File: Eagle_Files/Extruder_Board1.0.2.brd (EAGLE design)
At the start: 39.6 x 46.5 mm, 22 parts, among them J1 10118192-0001LF, U1 CP2102N-A01-GQFN20

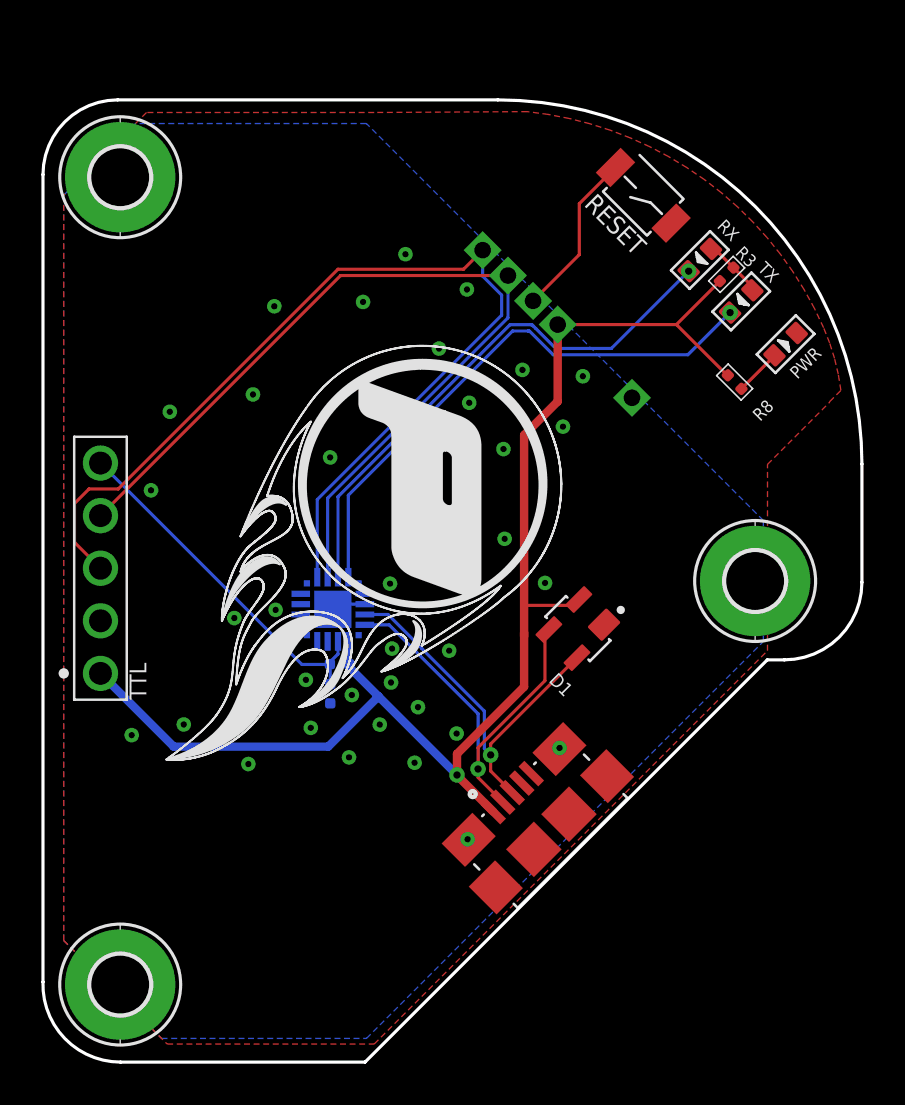
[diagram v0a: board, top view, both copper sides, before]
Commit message: pulled latest fixes from master
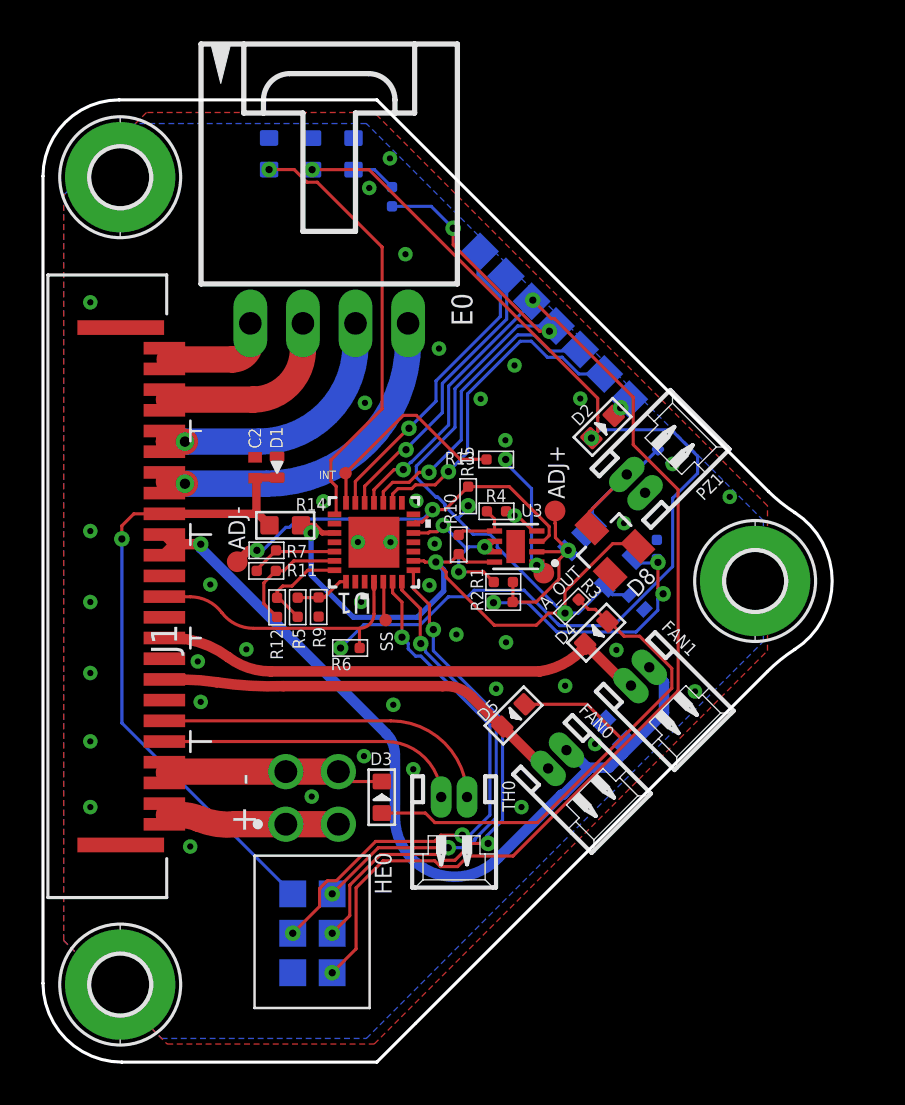
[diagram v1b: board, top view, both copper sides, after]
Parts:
- removed RESET: (no value), PiezoFFC:SEEED-SWITCH_SW2-2.6-3.0X2.5X1.2+0.4MM
- removed RX, TX: (no value), PiezoFFC:SEEED-LED_LED-0603
- removed TTL: JST-2.54MM_5P-2.54JST_2.54MM_5P_F, PiezoFFC:HDRVR5W64P254_1X5_1270X254X575B
- removed U$2: (no value), PiezoFFC:LOGO-PYR0BALL-SS-20MM
- added 5V, MISO, MOSI, RST, SCK: TPTP13SQ, PiezoFFC:TP13SQ
- added ADJ+, ADJ-, A_OUT: TPTP10R, PiezoFFC:TP10R
- added C1, C2: 0.1uF, PiezoFFC:CAPC1005X50
- added C3: 1uF, PiezoFFC:CAPC1609X80
- added D2, D3, D4, D5, ERR, TRG: (no value), PiezoFFC:SEEED-LED_LED-0603
- added D8: BAV199, PiezoFFC:SOT23
- added E0: C-GRID-04-70553, PiezoFFC:70553-04
- added FAN0, FAN1, PZ1, TH0: CON-MOLEX-2P-1.27MM048, PiezoFFC:53048-02
- added HE0: JST-2.54-2X2JST-DUPONT-2.54-2X2, PiezoFFC:HDRRAR4W64P254_2X2_556X736X556B
- added INT, SS: TPTP06R, testpad:TP06R
- added R10, R4: 10K, PiezoFFC:R0402
- added R11, R7: 220R, PiezoFFC:R0402
- added R12, R5: 330R, PiezoFFC:R0402
- added R13: 100R, PiezoFFC:R0402
- added R14: 0R, PiezoFFC:SEEED-RESISTOR_R0603
- added R15: 680R, PiezoFFC:R0402
- added R17: 3.3K, PiezoFFC:R0402
- added R19: 1M, PiezoFFC:R0402
- added R6: (no value), PiezoFFC:R0402
- added R9: 470R, PiezoFFC:R0402
- added SCL, SDA, ⏚: TPTP13SQ, testpad:TP13SQ
- added U2: MCP6001T-I/OTSOT-23-5_MC-L, PiezoFFC:SOT-23-5_MC-L
- added U3: LM358PWRDFN-8, PiezoFFC:SON50P200X200X60-9N
- +5V, GND, RST., RXD, TXD: value TP -> TPTP13SQ; device PiezoFFC:TP13SQ-HOLE -> testpad:TP13SQ
- D1: value SP0503BAHTG -> 1N4148DFN-1006-2; device PiezoFFC:SOT143 -> PiezoFFC:DIOC1006X70
- J1: value 10118192-0001LF -> SFW24R-1STE1LF; device PiezoFFC:AMPHENOL_10118192-0001LF -> PiezoFFC:CON24_1X24_DRB_SFW
- R1: value 22K -> 1M
- R2: value 47K -> 10K
- R3, R8: value (none) -> 1K
- U1: value CP2102N-A01-GQFN20 -> ATMEGA48PA-MMHR28M1-L; device PiezoFFC:SILABS_QFN20 -> PiezoFFC:28M1-L
- moved PWR 22.8 mm to (15.0, 44.0), flipped to the bottom, turned to 90 degrees
- moved R8 18.8 mm to (16.9, 41.9), flipped to the bottom, turned to 180 degrees
- moved R3 17.7 mm to (25.5, 22.1)
- moved J1 17.2 mm to (8.62, 23.1), turned to 90 degrees
- moved D1 16.5 mm to (11.3, 28.9), turned to 90 degrees
- moved R2 9.45 mm to (22.2, 22.4), flipped to the top, turned to 90 degrees
- moved R1 8.85 mm to (22.2, 23.3), flipped to the top, turned to 90 degrees
- moved U$1 4.51 mm to (15.0, 25.0), flipped to the bottom, turned to 0 degrees
- moved U1 3.80 mm to (16.0, 25.2), flipped to the top
- moved GND 0.15 mm to (28.3, 32.2)
- moved TXD 0.14 mm to (21.1, 39.3)
- moved +5V 0.11 mm to (24.8, 35.7)
- moved RXD 0.10 mm to (22.4, 38.1)
- moved RST. 0.07 mm to (23.6, 36.9)
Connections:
- removed net 5V_DC: +5V.TP, D1.2, J1.1, R1.2, R3.1, R8.1, TTL.1, U1.7
- removed net D+: D1.4, J1.3, U1.4
- removed net D-: D1.3, J1.2, U1.5
- removed net RXD: RXD.TP, TTL.4, U1.18
- removed net RXT: RX.-, U1.19
- removed net TXD: TTL.3, TXD.TP, U1.17
- removed net TXT: TX.-, U1.20
- removed net VBUS: R1.1, R2.2, TTL.5, U1.8
- removed net VDD: U1.6
- new net +5V: +5V.TP, C1.1, D8.2, R10.2, R14.2, R15.1, R3.1, R8.1, U1.16, U1.3, U2.5, U3.8
- new net COMP-: ADJ+.TP, R1.2, R2.2, U2.1, U3.2
- new net E0_1A: E0.3, J1.5, J1.6
- new net E0_1B: E0.4, J1.7, J1.8
- new net E0_2A: E0.2, J1.3, J1.4
- new net E0_2B: E0.1, J1.1, J1.2
- new net ERR_LED: ERR.+, U1.1
- new net FAN0_GATE: D5.-, FAN0.1, J1.17
- new net FAN1_GATE: D4.-, FAN1.1, J1.15
- new net GAIN_FB: R17.2, R2.1, U2.4
- new net HE0-: D3.-, HE0.3, HE0.4, J1.21, J1.22
- new net PZ+: D8.3, PZ1.2, R19.2, U2.3
- new net PZ_AMP_OUT: A_OUT.TP, R13.1, U3.1
- new net SCL: SCL.TP, U1.24
- new net SDA: SDA.TP, U1.23
- new net SPI_MISO: MISO.TP, U1.14
- new net SPI_MOSI: MOSI.TP, U1.13
- new net SPI_SCK: SCK.TP, U1.15
- new net SPI_SS: SS.TP, U1.12
- new net TH0+: J1.20, TH0.1
- new net TH0-: J1.19, TH0.2
- new net TRG_LED: D2.+, R6.2, TRG.+
- new net TTL_RXD: RXD.TP, U1.26
- new net TTL_TXD: TXD.TP, U1.27
- new net VADJ_R0: R11.2, R7.1, U1.5
- new net VADJ_R1: R11.1, R12.2, U1.6
- new net VADJ_R2: R12.1, R5.2, U1.7
- new net VADJ_R3: R5.1, R9.2, U1.8
- new net VADJ_SENSE: ADJ-.TP, R15.2, R7.2, U1.20, U3.3
- new net VCC: HE0.1, HE0.2, J1.23, J1.24
- new net VCC_REG: 5V.TP, C2.2, D1.C, J1.9, R14.1
- new net VREF_IN: R10.1, R4.2, U3.5
- new net V_FOLLOW: R1.1, U1.19, U3.6, U3.7
- new net V_INT: C3.1, FAN0.2, FAN1.2, J1.10, J1.11
- new net Z_MIN_TRIG: J1.13, R6.1, U1.11
- new net Z_TRG: INT.TP, R13.2, U1.28
- net GND: now also C1.2, C2.1, C3.2, D1.A, D2.-, D8.1, ERR.-, J1.12, J1.14, J1.16, J1.18, J1.25, J1.26, PZ1.1, R17.1, R19.1, R4.1, R9.1, TRG.-, U1.18, U1.29, U1.4, U2.2, U3.4, ⏚.TP; no longer D1.1, J1.5, J1.SH1, J1.SH2, J1.SH3, J1.SH4, J1.SH5, J1.SH6, R2.1, RESET.1, TTL.2, U1.12, U1.21, U1.3
- net LED_VCC: now also D3.+, D4.+, D5.+; no longer RX.+, TX.+
- net RST: now also RST.TP, U1.25; no longer RESET.2
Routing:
- net +5V: track 0.00 -> 68.3 mm, vias 0 -> 6
- net 5V_DC: track 67.7 -> 0.00 mm, vias 1 -> 0
- net RST: track 8.10 -> 59.5 mm, vias 0 -> 3
- net TRG_LED: track 0.00 -> 51.2 mm, vias 0 -> 3
- net TXD: track 48.3 -> 0.00 mm
- net RXD: track 42.7 -> 0.00 mm
- net V_INT: track 0.00 -> 40.8 mm, vias 0 -> 1
- net VCC_REG: track 0.00 -> 31.7 mm, vias 0 -> 1
- net TXT: track 27.0 -> 0.00 mm, vias 1 -> 0
- net RXT: track 26.3 -> 0.00 mm, vias 1 -> 0
- net LED_VCC: track 3.03 -> 29.1 mm
- net SPI_MOSI: track 0.00 -> 25.8 mm, vias 0 -> 3
- net SPI_SCK: track 0.00 -> 25.7 mm, vias 0 -> 3
- net FAN1_GATE: track 0.00 -> 24.1 mm
- net SPI_MISO: track 0.00 -> 22.8 mm, vias 0 -> 3
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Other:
- board size 39.6 x 46.5 mm -> 38.1 x 46.5 mm
- board text added: "+ -"
- board text added: "2B 2A 1A 1B"
- board text added: "Fan0"
- board text added: "Fan1"
- board text added: "HE0"
- board text added: "PZ1"
- board text added: "TH0"
- board text removed: "- +"
